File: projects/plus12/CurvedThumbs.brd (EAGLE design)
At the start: 123.2 x 54 mm, 15 parts

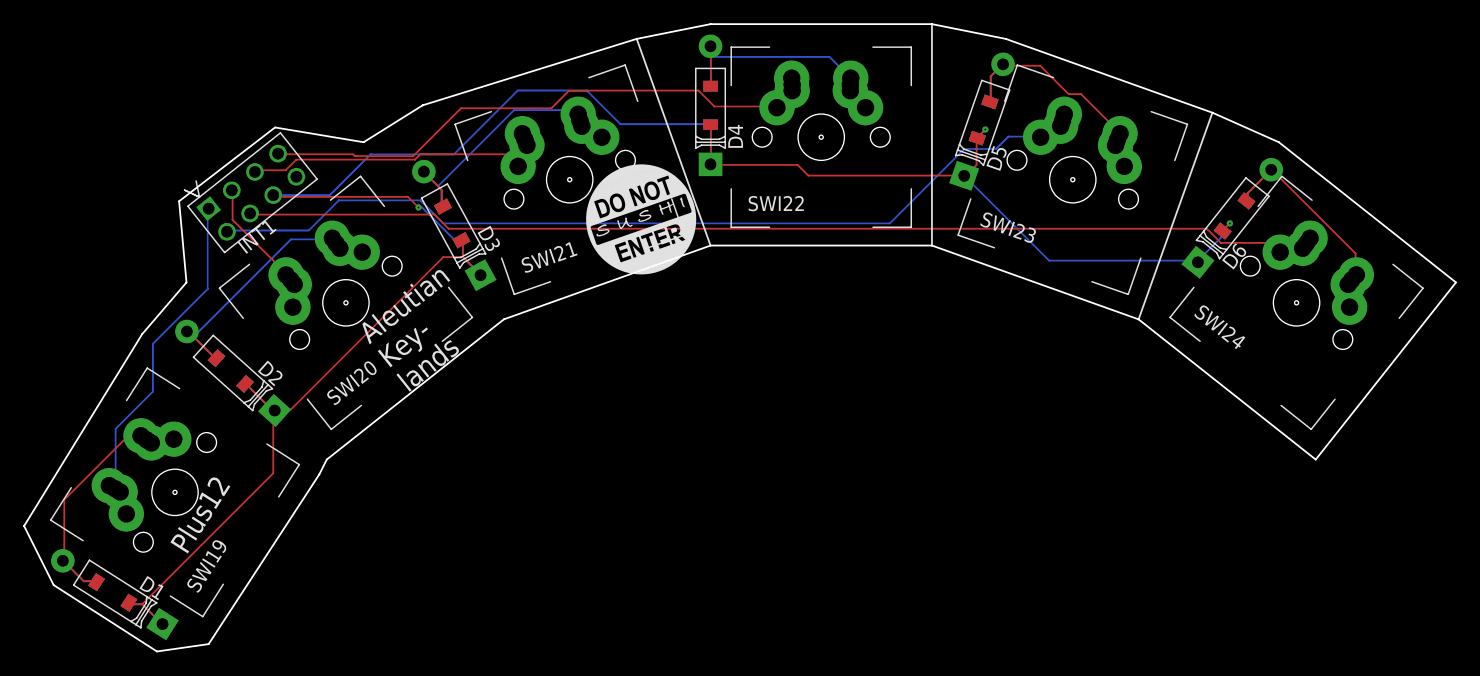
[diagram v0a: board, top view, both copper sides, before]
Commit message: more updates than should be in one commit, lots of work
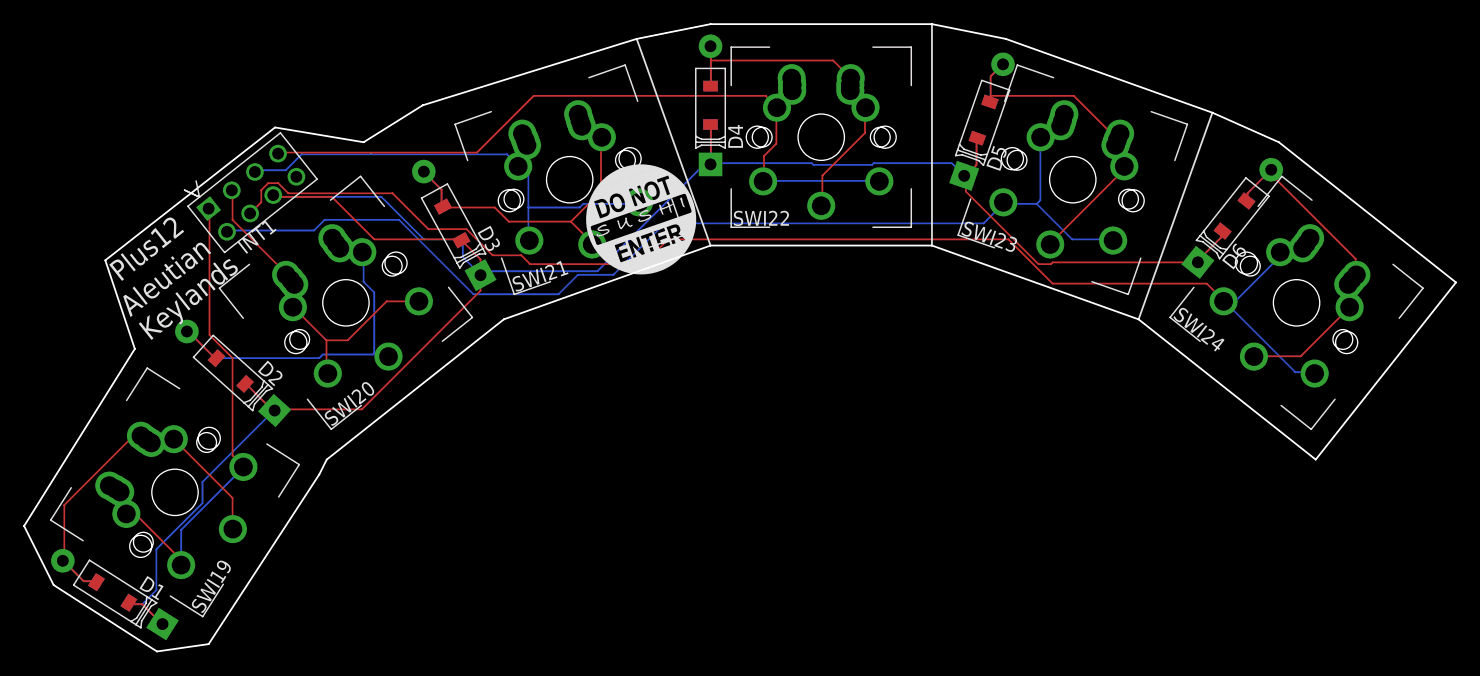
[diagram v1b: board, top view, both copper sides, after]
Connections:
- net N$1: now also SWI19.RLMID
- net N$10: now also SWI22.LLP, SWI22.LRLP
- net N$11: now also SWI23.LLP, SWI23.LRLP
- net N$12: now also SWI24.LLP, SWI24.LRLP
- net N$2: now also SWI20.RLMID
- net N$3: now also SWI21.RLMID
- net N$4: now also SWI22.RLMID
- net N$5: now also SWI23.RLMID
- net N$6: now also SWI24.RLMID
- net N$7: now also SWI19.LLP, SWI19.LRLP
- net N$8: now also SWI20.LLP, SWI20.LRLP
- net N$9: now also SWI21.LLP, SWI21.LRLP
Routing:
- net N$12: track 93.6 -> 113.4 mm
- net N$9: track 28.7 -> 45.6 mm
- net N$10: track 50.0 -> 66.0 mm
- net N$8: track 14.5 -> 29.9 mm
- net N$11: track 79.3 -> 94.3 mm
- net N$6: track 20.3 -> 34.6 mm
- net N$1: track 21.5 -> 35.8 mm
- net N$4: track 20.6 -> 34.3 mm
- net N$7: track 31.8 -> 44.9 mm
- net N$5: track 21.1 -> 34.1 mm
- net N$3: track 22.4 -> 34.7 mm
- net N$2: track 23.2 -> 35.0 mm
- net N$13: track 188.8 -> 194.3 mm, vias 3 -> 0
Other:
- outline, holes or cut-outs redrawn
- board text added: "Aleutian Keylands"
- board text removed: "Aleutian Key- lands"

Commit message: more updates than should be in one commit, lots of work
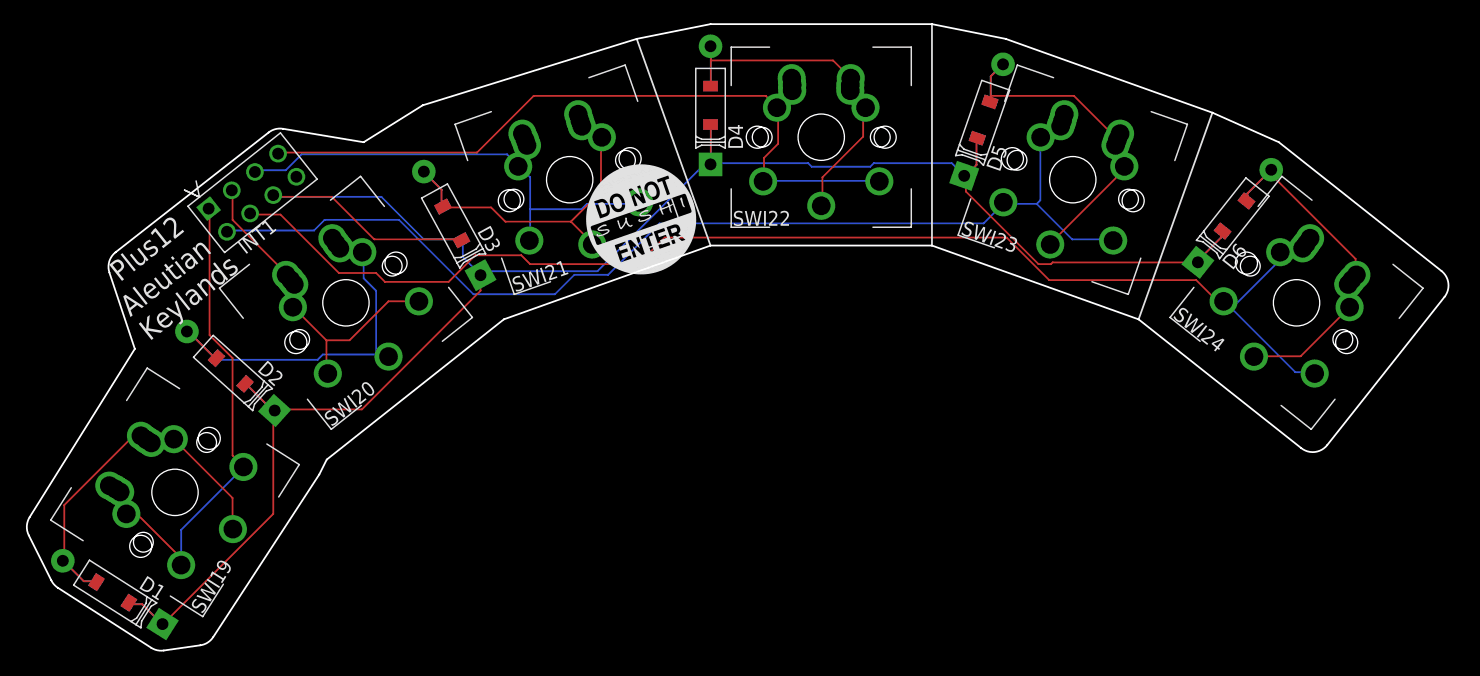
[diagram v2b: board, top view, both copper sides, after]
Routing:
- net N$13: track 194.3 -> 191.6 mm
- net N$2: track 35.0 -> 36.4 mm
- net N$12: track 113.4 -> 112.9 mm
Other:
- board size 123.2 x 54 mm -> 122.3 x 53.9 mm
